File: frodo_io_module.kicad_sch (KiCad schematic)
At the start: 2 parts, among them J1 Molex MicroFit 2x3, J2 Molex MicroFit 2x3

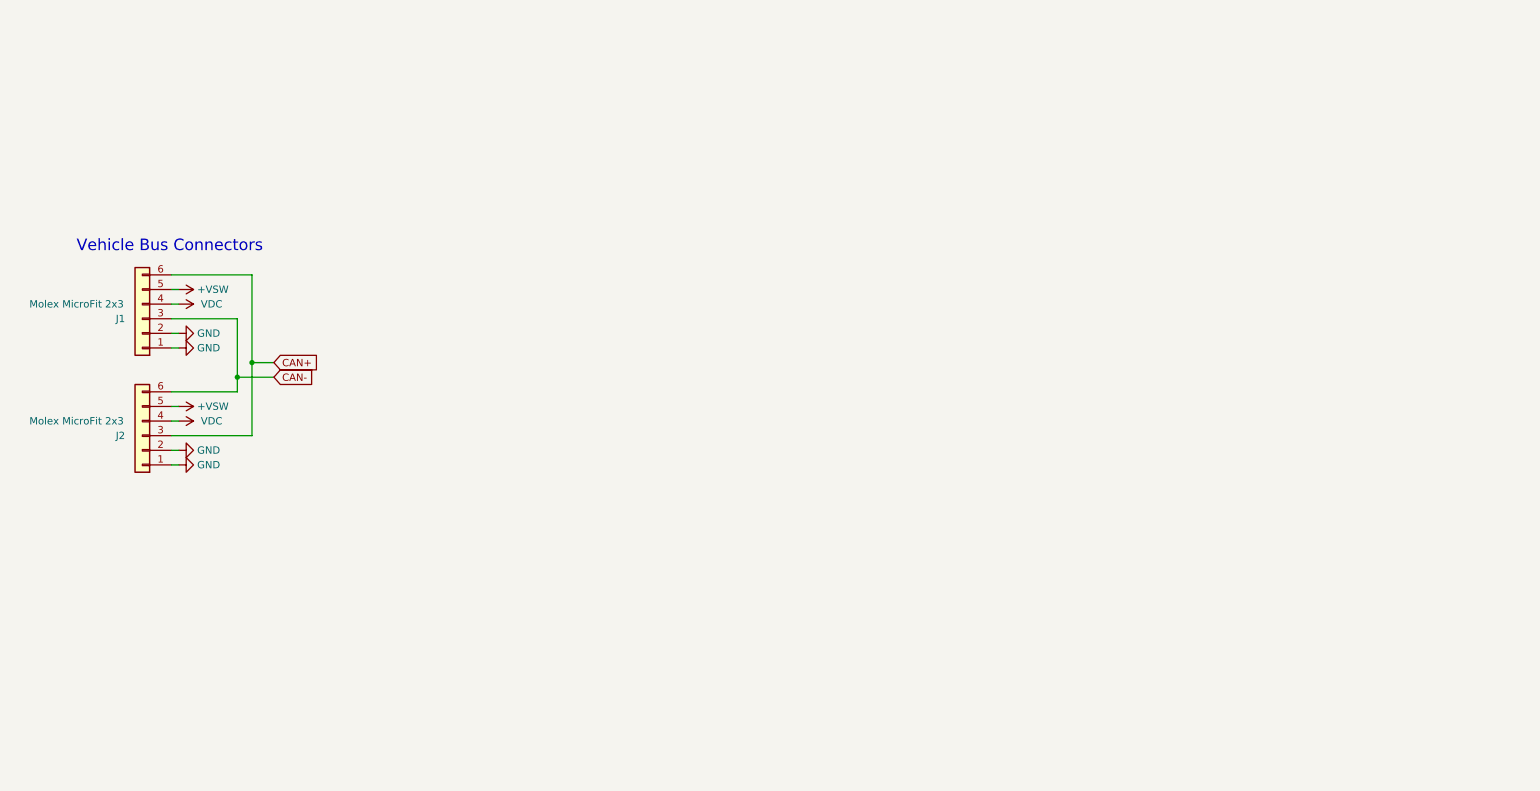
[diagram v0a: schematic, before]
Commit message: basic microcontroller peripherals
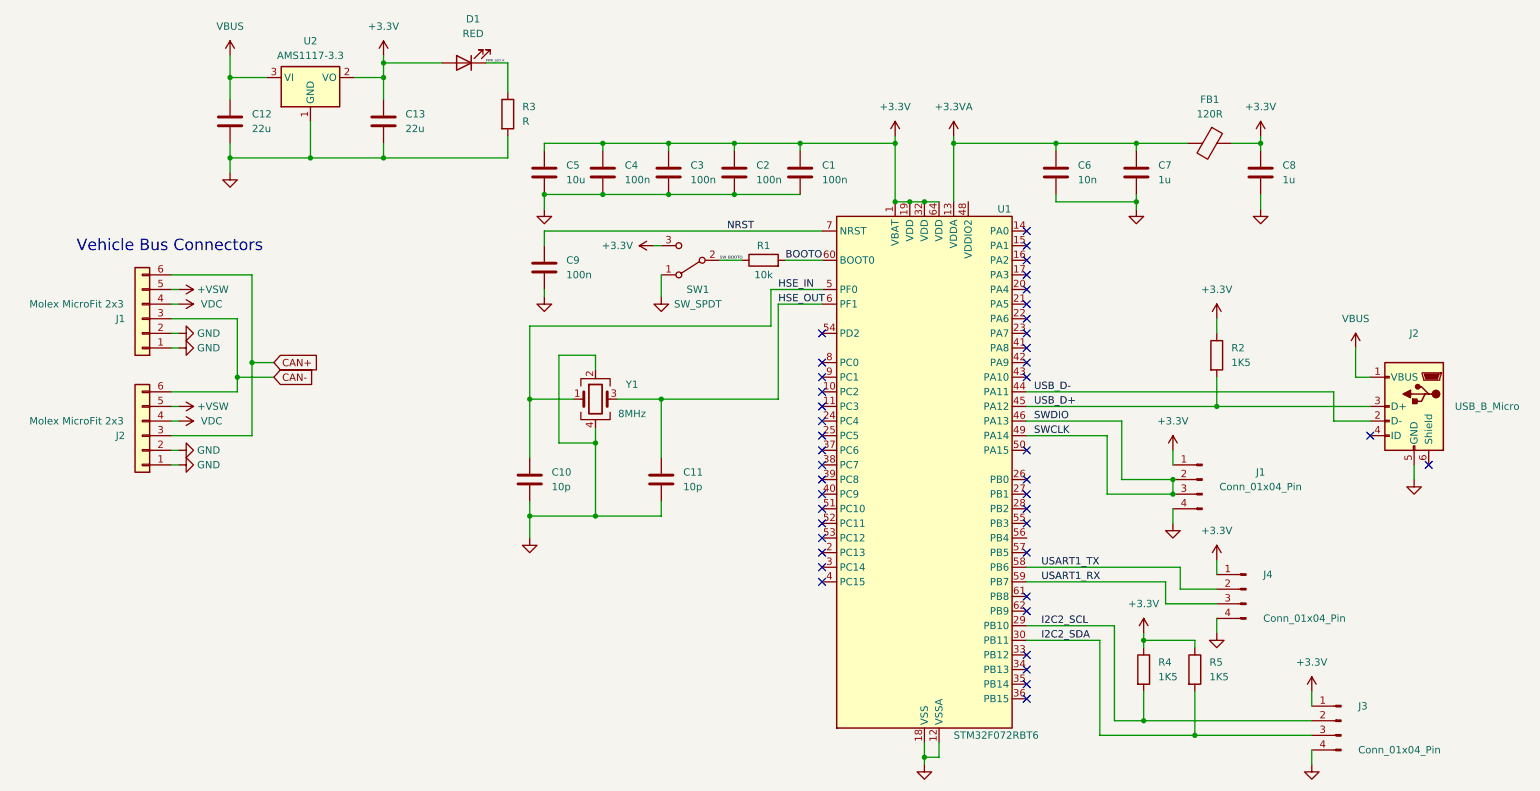
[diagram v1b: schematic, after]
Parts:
- added C1, C2, C3, C4, C9: 100n, symbol Device:C
- added C10, C11: 10p, symbol Device:C
- added C12, C13: 22u, symbol Device:C
- added C5: 10u, symbol Device:C
- added C6: 10n, symbol Device:C
- added C7, C8: 1u, symbol Device:C
- added D1: RED, symbol Device:LED
- added FB1: 120R, symbol Device:FerriteBead
- added J1, J3, J4: Conn_01x04_Pin, symbol Connector:Conn_01x04_Pin
- added J2: USB_B_Micro, symbol Connector:USB_B_Micro
- added R1: 10k, symbol Device:R
- added R2, R4, R5: 1K5, symbol Device:R
- added R3: R, symbol Device:R
- added SW1: SW_SPDT, symbol Switch:SW_SPDT
- added U1: STM32F072RBT6, Package_QFP:LQFP-64_10x10mm_P0.5mm, symbol MCU_ST_STM32F0:STM32F072RBTx
- added U2: AMS1117-3.3, Package_TO_SOT_SMD:SOT-223-3_TabPin2, symbol Regulator_Linear:AMS1117-3.3
- added Y1: 8MHz, symbol Device:Crystal_GND24
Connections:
- net GND: now also C1.2, C10.2, C11.2, C12.2, C13.2, C2.2, C3.2, C4.2, C5.2, C6.2, C7.2, C8.2, C9.2, J1.4 (Pin_4), J2.5 (GND), J3.4 (Pin_4), J4.4 (Pin_4), R3.2, SW1.1 (A), U1.12 (VSSA), U1.18 (VSS), U1.31 (VSS), U1.47 (VSS), U1.63 (VSS), U2.1 (GND), Y1.2, Y1.4
- new net +3.3V: C1.1, C13.1, C2.1, C3.1, C4.1, C5.1, C8.1, D1.2 (A), FB1.1, J1.1 (Pin_1), J3.1 (Pin_1), J4.1 (Pin_1), R2.1, R4.1, R5.1, SW1.3 (C), U1.1 (VBAT), U1.19 (VDD), U1.32 (VDD), U1.64 (VDD), U2.2 (VO)
- new net +3.3VA: C6.1, C7.1, FB1.2, U1.13 (VDDA)
- new net BOOTO: R1.2, U1.60 (BOOT0)
- new net HSE_IN: C10.1, U1.5 (PF0), Y1.1
- new net HSE_OUT: C11.1, U1.6 (PF1), Y1.3
- new net I2C2_SCL: J3.2 (Pin_2), R4.2, U1.29 (PB10)
- new net I2C2_SDA: J3.3 (Pin_3), R5.2, U1.30 (PB11)
- new net NRST: C9.1, U1.7 (NRST)
- new net PWR_LED_K: D1.1 (K), R3.1
- new net SWCLK: J1.2 (Pin_2), J1.3 (Pin_3), U1.46 (PA13), U1.49 (PA14)
- new net SW_BOOTO: R1.1, SW1.2 (B)
- new net USART1_RX: J4.3 (Pin_3), U1.59 (PB7)
- new net USART1_TX: J4.2 (Pin_2), U1.58 (PB6)
- new net USB_D+: J2.3 (D+), R2.2, U1.45 (PA12)
- new net USB_D-: J2.2 (D-), U1.44 (PA11)
- new net VBUS: C12.1, J2.1 (VBUS), U2.3 (VI)
- no-connect marks 0 -> 42
